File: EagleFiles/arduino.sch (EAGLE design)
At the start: 22 parts, among them IC2 74250N, IC3 74250N, IC4 74250N, J1 AVR_SPI, U1 ATMEGA168

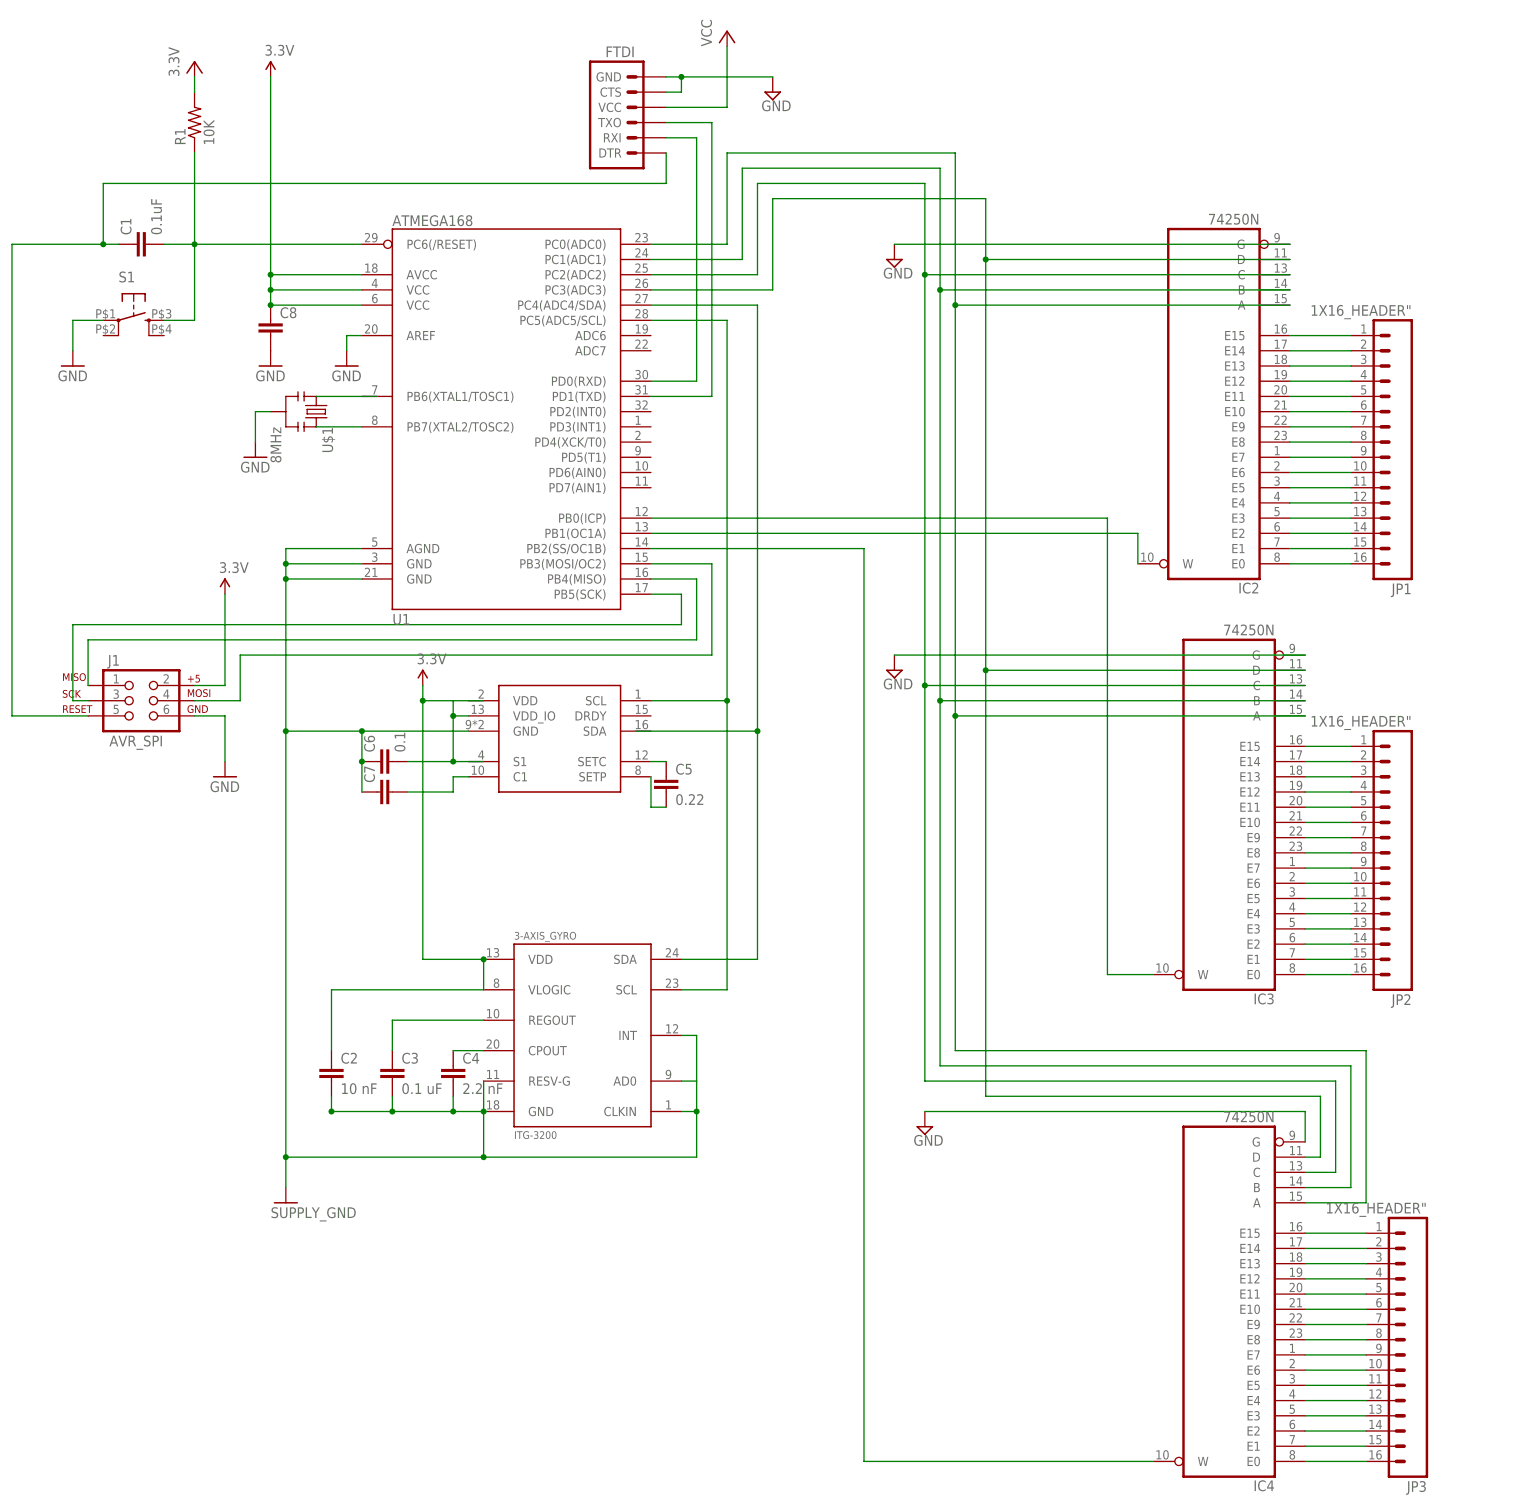
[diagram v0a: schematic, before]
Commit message: finished first rev
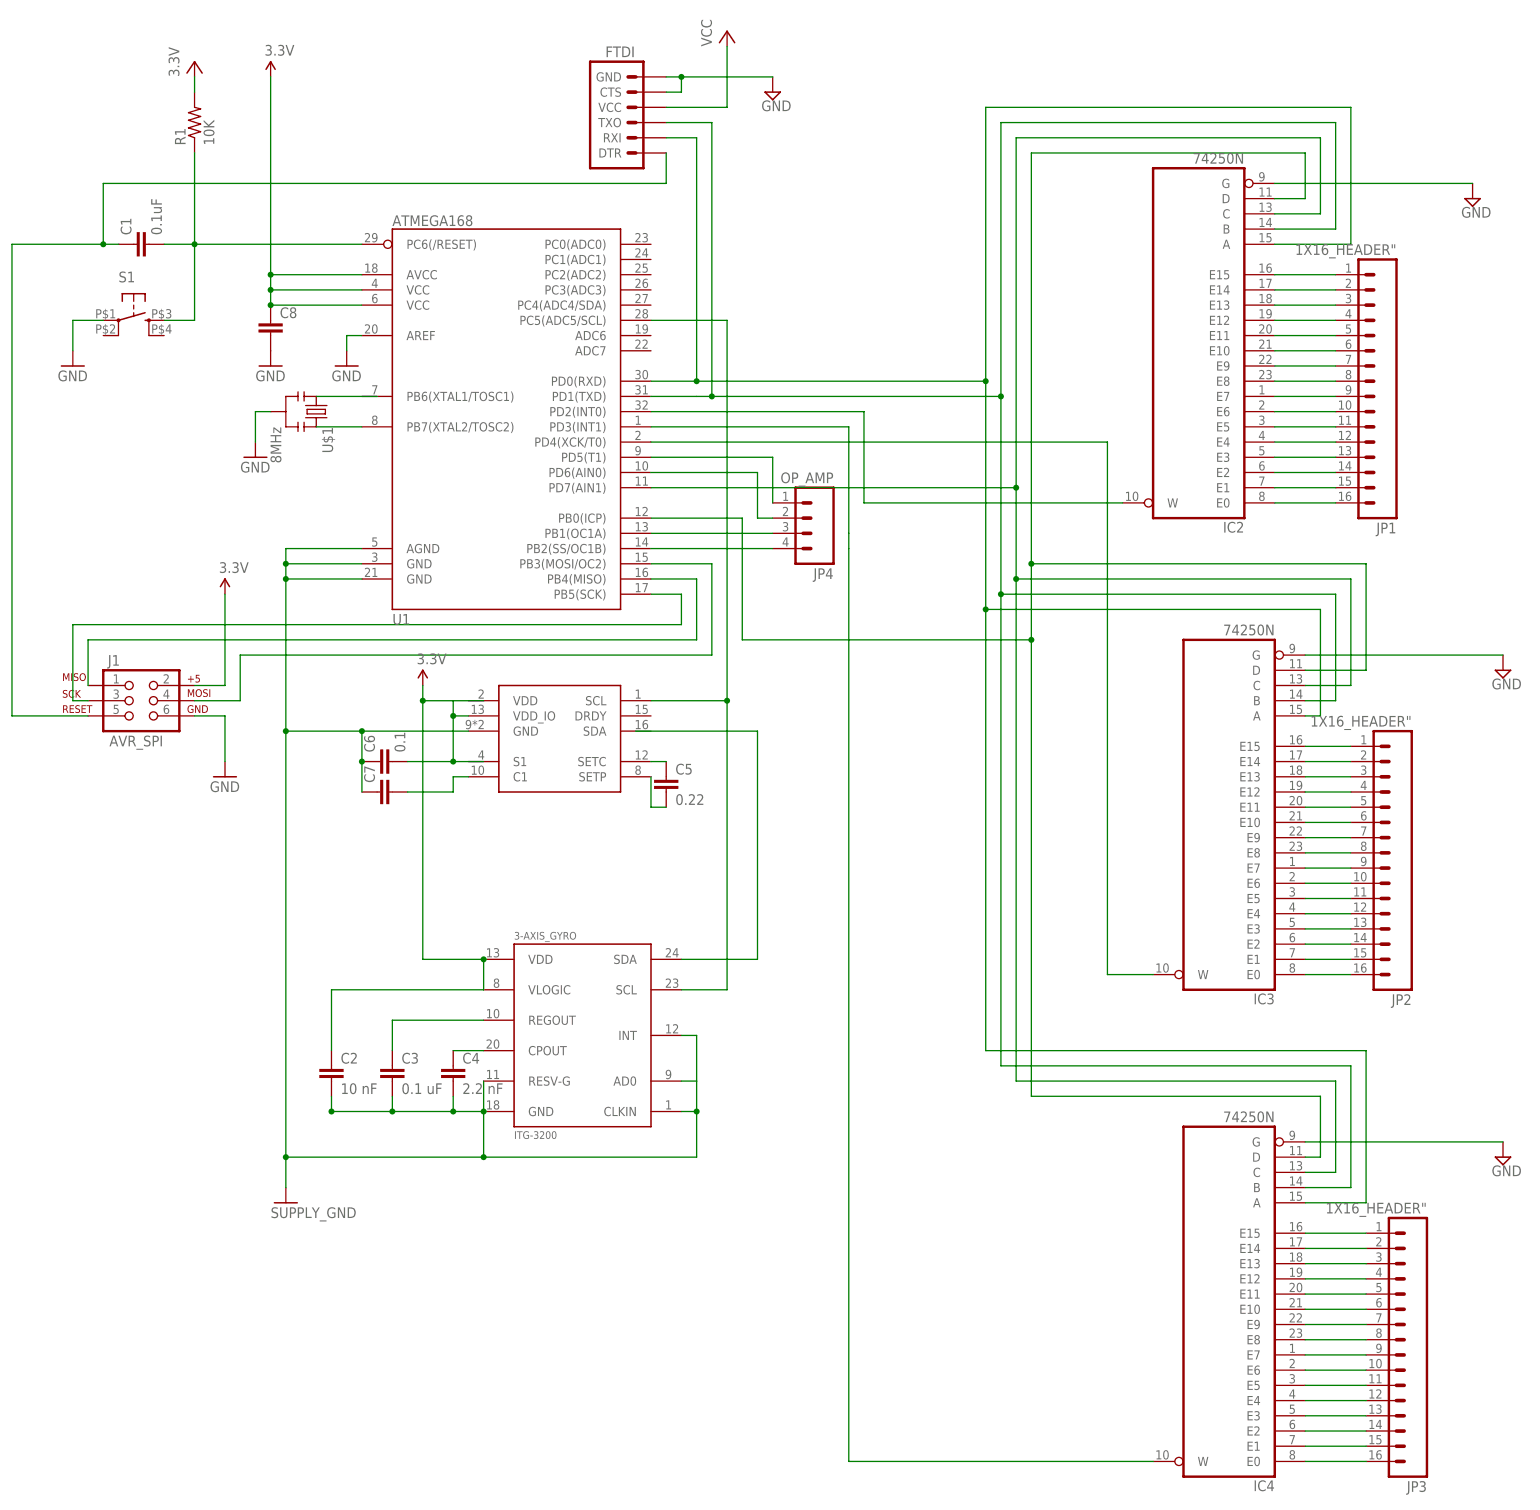
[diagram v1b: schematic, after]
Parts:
- added JP4: OP_AMP, RBBB:1X04_HEADER"
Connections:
- removed net N$3: IC2A.B, IC3A.B, IC4A.B, U1.PC1(ADC1)
- removed net N$4: IC2A.A, IC3A.A, IC4A.A, U1.PC0(ADC0)
- new net N$72: JP4.3, U1.PB1(OC1A)
- new net N$73: JP4.1, U1.PD5(T1)
- new net N$74: JP4.2, U1.PD6(AIN0)
- new net N$75: JP4.4, U1.PB2(SS/OC1B)
- net N$2: now also U1.PD7(AIN1); no longer U1.PC2(ADC2)
- net N$42: now also U1.PD3(INT1); no longer U1.PB2(SS/OC1B)
- net N$43: no longer U1.PC4(ADC4/SDA)
- net N$5: now also U1.PD2(INT0); no longer U1.PB1(OC1A)
- net N$6: now also U1.PD4(XCK/T0); no longer U1.PB0(ICP)
- net N$63: now also IC2A.A, IC3A.A, IC4A.A
- net N$66: now also IC2A.B, IC3A.B, IC4A.B
- net N$7: now also U1.PB0(ICP); no longer U1.PC3(ADC3)
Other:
- moved on the sheet: IC2, JP1
